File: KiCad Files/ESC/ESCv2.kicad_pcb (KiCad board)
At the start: 2 copper layers, 0 parts

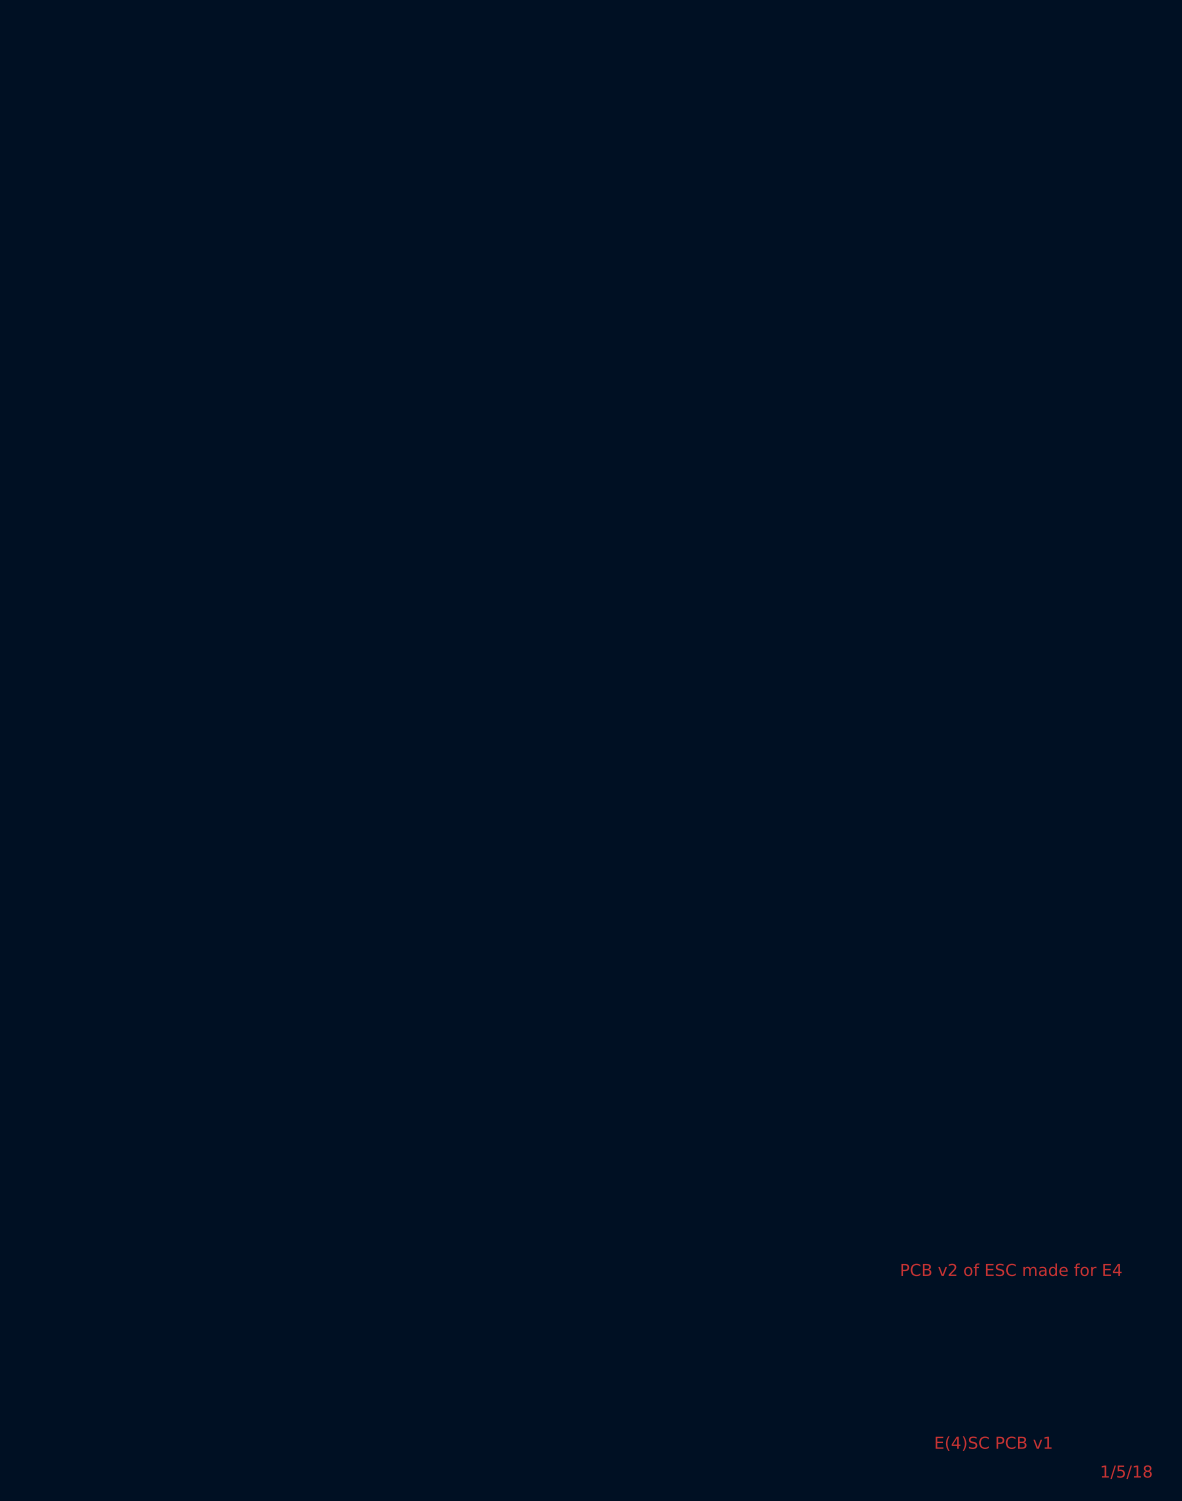
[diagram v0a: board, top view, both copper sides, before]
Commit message: Added PCB v2 and reorganized code
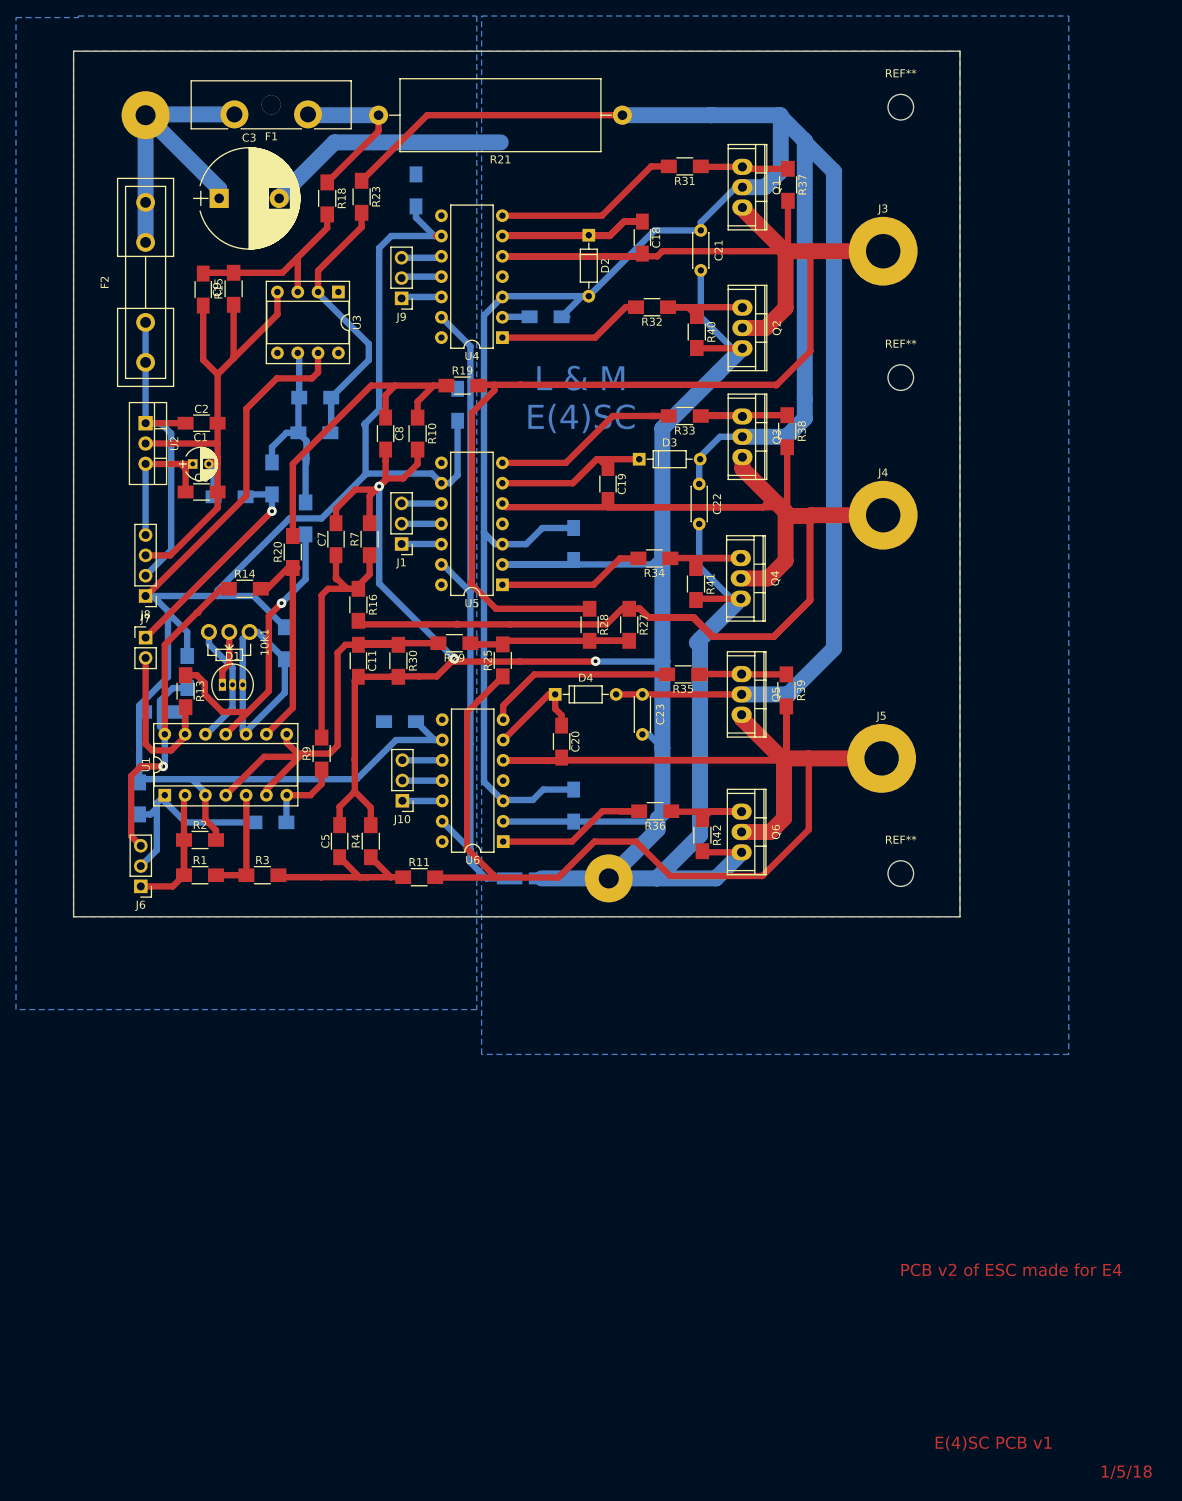
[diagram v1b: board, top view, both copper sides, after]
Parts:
- added 10k1: POT_TRIM, Potentiometers:Potentiometer_WirePads_Small, F.Cu at (101.4, 88.2)
- added BT1: Battery, Wire_Connections_Bridges:WireConnection_2.50mmDrill_LargePad, F.Cu at (152.5, 141.4)
- added C1: 1u, Capacitors_THT:CP_Radial_D4.0mm_P2.00mm, F.Cu at (94.3, 67.2)
- added C10: 5.6n, Capacitors_SMD:C_1206_HandSoldering, B.Cu at (109.5, 63.3)
- added C11: 6.8n, Capacitors_SMD:C_1206_HandSoldering, F.Cu at (115.0, 91.8)
- added C12: 10n, Capacitors_SMD:C_1206_HandSoldering, B.Cu at (122.2, 33.0)
- added C13: 10n, Capacitors_SMD:C_1206_HandSoldering, B.Cu at (127.4, 59.8)
- added C14: 10n, Capacitors_SMD:C_1206_HandSoldering, B.Cu at (120.2, 99.4)
- added C15: 33n, Capacitors_SMD:C_1206_HandSoldering, B.Cu at (138.4, 48.8)
- added C16: 33n, Capacitors_SMD:C_1206_HandSoldering, B.Cu at (141.9, 77.2)
- added C17: 33n, Capacitors_SMD:C_1206_HandSoldering, B.Cu at (141.9, 109.9)
- added C18: 1u, Capacitors_SMD:C_1206_HandSoldering, F.Cu at (150.5, 38.9)
- added C19: 1u, Capacitors_SMD:C_1206_HandSoldering, F.Cu at (146.2, 69.7)
- added C2: 100n, Capacitors_SMD:C_1206_HandSoldering, F.Cu at (95.4, 62.1)
- added C20: 1u, Capacitors_SMD:C_1206_HandSoldering, F.Cu at (140.4, 101.9)
- added C21: 1u, Capacitors_THT:C_Disc_D4.3mm_W1.9mm_P5.00mm, F.Cu at (157.8, 38.0)
- added C22: 1u, Capacitors_THT:C_Disc_D4.3mm_W1.9mm_P5.00mm, F.Cu at (157.6, 69.7)
- added C23: 1u, Capacitors_THT:C_Disc_D4.3mm_W1.9mm_P5.00mm, F.Cu at (150.5, 96.0)
- added C3: 330u, Capacitors_THT:CP_Radial_D12.5mm_P7.50mm, F.Cu at (97.6, 34.0)
- added C4: 33n, Capacitors_SMD:C_1206_HandSoldering, B.Cu at (98.9, 71.3)
- added C5: 1n, Capacitors_SMD:C_1206_HandSoldering, F.Cu at (112.7, 114.3)
- added C6: 1n, Capacitors_SMD:C_1206_HandSoldering, F.Cu at (95.4, 70.7)
- added C7: 1n, Capacitors_SMD:C_1206_HandSoldering, F.Cu at (112.2, 76.6)
- added C8: 1n, Capacitors_SMD:C_1206_HandSoldering, F.Cu at (118.4, 63.4)
- added C9: 5.6n, Capacitors_SMD:C_1206_HandSoldering, F.Cu at (95.6, 45.4)
- added D1: TL431LP, TO_SOT_Packages_THT:TO-92_Inline_Narrow_Oval, F.Cu at (98.0, 94.8)
- added D2: IN4148, Diodes_THT:D_DO-35_SOD27_P7.62mm_Horizontal, F.Cu at (143.8, 38.6)
- added D3: IN4148, Diodes_THT:D_DO-35_SOD27_P7.62mm_Horizontal, F.Cu at (150.1, 66.6)
- added D4: IN4148, Diodes_THT:D_DO-35_SOD27_P7.62mm_Horizontal, F.Cu at (139.6, 96.0)
- added F1: Fuse, Fuse_Holders_and_Fuses:Fuseholder_ATO_Blade_littlefuse_Pudenz_2_Pin, F.Cu at (108.7, 23.5)
- added F2: Fuse, Fuse_Holders_and_Fuses:Fuseholder5x20_horiz_open_inline_Type-I, F.Cu at (88.4, 54.5)
- added J1: Conn_01x03, Socket_Strips:Socket_Strip_Straight_1x03_Pitch2.54mm, F.Cu at (120.4, 77.2)
- added J10: Conn_01x03, Socket_Strips:Socket_Strip_Straight_1x03_Pitch2.54mm, F.Cu at (120.5, 109.3)
- added J3: Conn_01x01, Mounting_Holes:MountingHole_4.3mm_M4_Pad, F.Cu at (180.6, 40.6)
- added J4: Conn_01x01, Mounting_Holes:MountingHole_4.3mm_M4_Pad, F.Cu at (180.6, 73.6)
- added J5: Conn_01x01, Mounting_Holes:MountingHole_4.3mm_M4_Pad, F.Cu at (180.4, 104.0)
- added J6: Conn_01x03, Socket_Strips:Socket_Strip_Straight_1x03_Pitch2.54mm, F.Cu at (87.8, 120.0)
- added J7: Conn_01x02, Socket_Strips:Socket_Strip_Straight_1x02_Pitch2.54mm, F.Cu at (88.4, 88.9)
- added J8: Conn_01x04, Socket_Strips:Socket_Strip_Straight_1x04_Pitch2.54mm, F.Cu at (88.4, 83.7)
- added J9: Conn_01x03, Socket_Strips:Socket_Strip_Straight_1x03_Pitch2.54mm, F.Cu at (120.4, 46.5)
- added JP1: Jumper_NC_Small, Capacitors_Tantalum_SMD:CP_Tantalum_Case-A_EIA-3216-18_Hand, B.Cu at (135.9, 119.0)
- added Q1: IRF3205, Power_Integrations:TO-220, F.Cu at (163.0, 32.6)
- added Q2: IRF3205, Power_Integrations:TO-220, F.Cu at (163.0, 50.2)
- added Q3: IRF3205, Power_Integrations:TO-220, F.Cu at (163.0, 63.8)
- added Q4: IRF3205, Power_Integrations:TO-220, F.Cu at (162.8, 81.5)
- added Q5: IRF3205, Power_Integrations:TO-220, F.Cu at (162.9, 96.0)
- added Q6: IRF3205, Power_Integrations:TO-220, F.Cu at (162.9, 113.2)
- added R1: 220k, Resistors_SMD:R_1206_HandSoldering, F.Cu at (95.2, 118.6)
- added R10: 100k, Resistors_SMD:R_1206_HandSoldering, F.Cu at (122.4, 63.4)
- added R11: 100k, Resistors_SMD:R_1206_HandSoldering, F.Cu at (122.6, 118.8)
- added R12: 6k8, Resistors_SMD:R_1206_HandSoldering, B.Cu at (90.2, 98.2)
- added R13: 220k, Resistors_SMD:R_1206_HandSoldering, F.Cu at (93.4, 95.6)
- added R14: 220k, Resistors_SMD:R_1206_HandSoldering, F.Cu at (100.8, 82.8)
- added R15: 33k, Resistors_SMD:R_1206_HandSoldering, F.Cu at (99.4, 45.3)
- added R16: 100k, Resistors_SMD:R_1206_HandSoldering, F.Cu at (115.0, 84.8)
- added R17: 6.8k, Resistors_SMD:R_1206_HandSoldering, B.Cu at (93.6, 93.2)
- added R18: 3k, Resistors_SMD:R_1206_HandSoldering, F.Cu at (111.1, 34.0)
- added R19: 100k, Resistors_SMD:R_1206_HandSoldering, F.Cu at (128.0, 57.4)
- added R2: 6.8k, Resistors_SMD:R_1206_HandSoldering, F.Cu at (95.2, 114.2)
- added R20: 10k, Resistors_SMD:R_1206_HandSoldering, F.Cu at (106.8, 78.2)
- added R21: 5m, Resistors_THT:R_Axial_Power_L25.0mm_W9.0mm_P30.48mm, F.Cu at (148.0, 23.6)
- added R22: 10k, Resistors_SMD:R_1206_HandSoldering, B.Cu at (108.4, 74.0)
- added R23: 3k, Resistors_SMD:R_1206_HandSoldering, F.Cu at (115.4, 33.8)
- added R24: 330, Resistors_SMD:R_1206_HandSoldering, B.Cu at (105.8, 89.6)
- added R25: 6k8, Resistors_SMD:R_1206_HandSoldering, F.Cu at (133.1, 91.8)
- added R26: 33k, Resistors_SMD:R_1206_HandSoldering, B.Cu at (109.6, 58.9)
- added R27: 6k8, Resistors_SMD:R_1206_HandSoldering, F.Cu at (148.8, 87.3)
- added R28: 6k8, Resistors_SMD:R_1206_HandSoldering, F.Cu at (143.9, 87.3)
- added R29: 100k, Resistors_SMD:R_1206_HandSoldering, F.Cu at (127.0, 89.6)
- added R3: 10k, Resistors_SMD:R_1206_HandSoldering, F.Cu at (103.0, 118.6)
- added R30: 100k, Resistors_SMD:R_1206_HandSoldering, F.Cu at (120.0, 91.8)
- added R31: 22, Resistors_SMD:R_1206_HandSoldering, F.Cu at (155.8, 30.0)
- added R32: 22, Resistors_SMD:R_1206_HandSoldering, F.Cu at (151.7, 47.6)
- added R33: 22, Resistors_SMD:R_1206_HandSoldering, F.Cu at (155.8, 61.2)
- added R34: 22, Resistors_SMD:R_1206_HandSoldering, F.Cu at (152.0, 79.0)
- added R35: 22, Resistors_SMD:R_1206_HandSoldering, F.Cu at (155.6, 93.5)
- added R36: 22, Resistors_SMD:R_1206_HandSoldering, F.Cu at (152.1, 110.6)
- added R37: 10k, Resistors_SMD:R_1206_HandSoldering, F.Cu at (168.7, 32.3)
- added R38: 10k, Resistors_SMD:R_1206_HandSoldering, F.Cu at (168.6, 63.1)
- added R39: 10k, Resistors_SMD:R_1206_HandSoldering, F.Cu at (168.5, 95.5)
- added R4: 100k, Resistors_SMD:R_1206_HandSoldering, F.Cu at (116.5, 114.3)
- added R40: 10k, Resistors_SMD:R_1206_HandSoldering, F.Cu at (157.3, 50.7)
- added R41: 10k, Resistors_SMD:R_1206_HandSoldering, F.Cu at (157.2, 82.2)
- added R42: 10k, Resistors_SMD:R_1206_HandSoldering, F.Cu at (158.0, 113.6)
- added R5: 220k, Resistors_SMD:R_1206_HandSoldering, B.Cu at (104.0, 112.0)
- added R6: 6.8k, Resistors_SMD:R_1206_HandSoldering, B.Cu at (87.6, 109.0)
- added R7: 100k, Resistors_SMD:R_1206_HandSoldering, F.Cu at (116.4, 76.6)
- added R8: 4k7, Resistors_SMD:R_1206_HandSoldering, B.Cu at (104.2, 69.0)
- added R9: 10k, Resistors_SMD:R_1206_HandSoldering, F.Cu at (110.4, 103.4)
- added REF**: MountingHole_3.2mm_M3, Mounting_Holes:MountingHole_3.2mm_M3, F.Cu at (182.8, 56.4)
- added REF**: MountingHole_3.2mm_M3, Mounting_Holes:MountingHole_3.2mm_M3, F.Cu at (182.8, 118.4)
- added REF**: MountingHole_3.2mm_M3, Mounting_Holes:MountingHole_3.2mm_M3, F.Cu at (182.8, 22.6)
- added U1: LM339, Housings_DIP:DIP-14_W7.62mm_Socket, F.Cu at (90.8, 108.6)
- added U2: L7809, TO_SOT_Packages_THT:TO-220-3_Vertical, F.Cu at (88.4, 62.1)
- added U3: MCP601-xP, Housings_DIP:DIP-8_W7.62mm_Socket, F.Cu at (112.5, 45.7)
- added U4: IR2110, Housings_DIP:DIP-14_W7.62mm, F.Cu at (133.0, 51.4)
- added U5: IR2110, Housings_DIP:DIP-14_W7.62mm, F.Cu at (133.0, 82.3)
- added U6: IR2110, Housings_DIP:DIP-14_W7.62mm, F.Cu at (133.1, 114.4)
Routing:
- net PowerGND: track 0.00 -> 387.7 mm, vias 0 -> 3
- net PowerVCC: track 0.00 -> 350.7 mm
- net LogicVCC: track 0.00 -> 235.6 mm
- net /PhaseB: track 0.00 -> 212.4 mm
- net /PhaseC: track 0.00 -> 206.8 mm
- net /PhaseA: track 0.00 -> 191.7 mm
- net LogicGND: track 0.00 -> 174.7 mm
- net NeutralPoint': track 0.00 -> 56.3 mm
- net /PhaseATrig: track 0.00 -> 49.2 mm, vias 0 -> 1
- net Net-(BT1-Pad1): track 0.00 -> 47.6 mm
- net /PhaseABEMF: track 0.00 -> 41.6 mm
- net BatVoltMeas: track 0.00 -> 40.4 mm
- net Net-(R13-Pad1): track 0.00 -> 39.6 mm, vias 0 -> 1
- net Net-(C18-Pad1): track 0.00 -> 36.5 mm
- net Net-(C10-Pad1): track 0.00 -> 34.4 mm
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- added copper zone on B.Cu, net LogicGND
- added copper zone on B.Cu, net PowerGND
- added copper zone on F.Cu, net PowerVCC
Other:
- board outline added: 110.8 x 108.2 mm
- net class Default: clearance 0.3 -> 0.01; trace_width 1.5 -> 0.8
- net class Power: clearance 0.6 -> 0.1
- rule trace_clearance: 0.3 -> 0.01
- board text added: "L & M E(4)SC"
